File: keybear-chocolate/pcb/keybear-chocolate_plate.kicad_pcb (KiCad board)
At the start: 2 copper layers, 151.4 x 117.1 mm, 33 parts, among them J1 MJ-4PP-9, SW10 SW_PUSH, SW11 SW_PUSH, SW12 SW_PUSH, SW13 SW_PUSH, SW14 SW_PUSH, SW15 SW_PUSH, SW16 SW_PUSH, SW17 SW_PUSH, SW18 SW_PUSH, SW19 SW_PUSH, SW2 KEY_SWITCH, SW2 SW_PUSH, SW20 SW_PUSH, SW21 SW_PUSH, SW22 SW_PUSH, SW23 SW_PUSH, SW24 Rotary_Encoder_Switch, SW3 SW_PUSH, SW4 SW_PUSH, SW5 SW_PUSH, SW6 SW_PUSH, SW7 SW_PUSH, SW8 SW_PUSH, SW9 SW_PUSH, U1 ProMicro

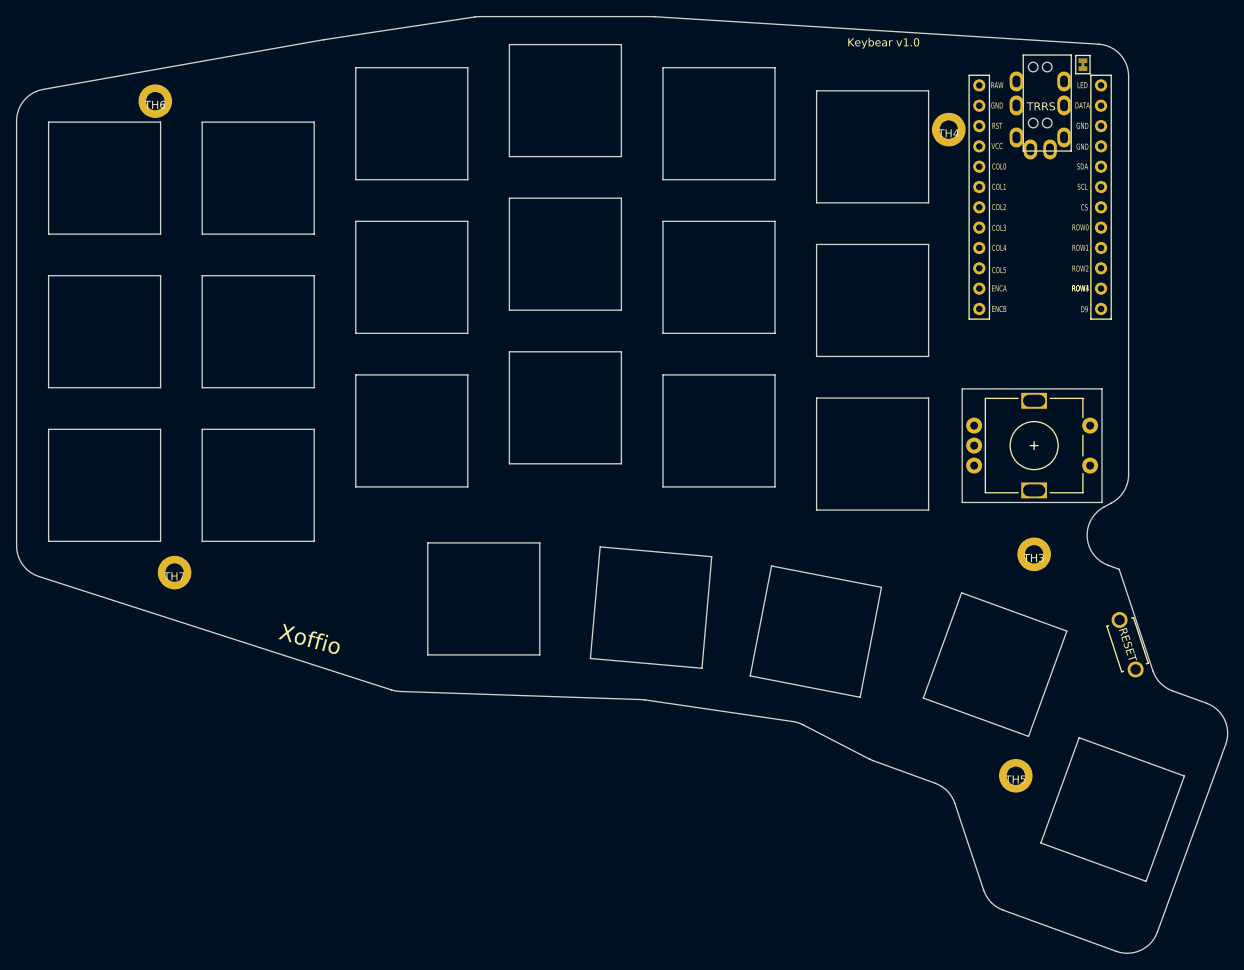
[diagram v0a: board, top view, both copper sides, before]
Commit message: updating the plate
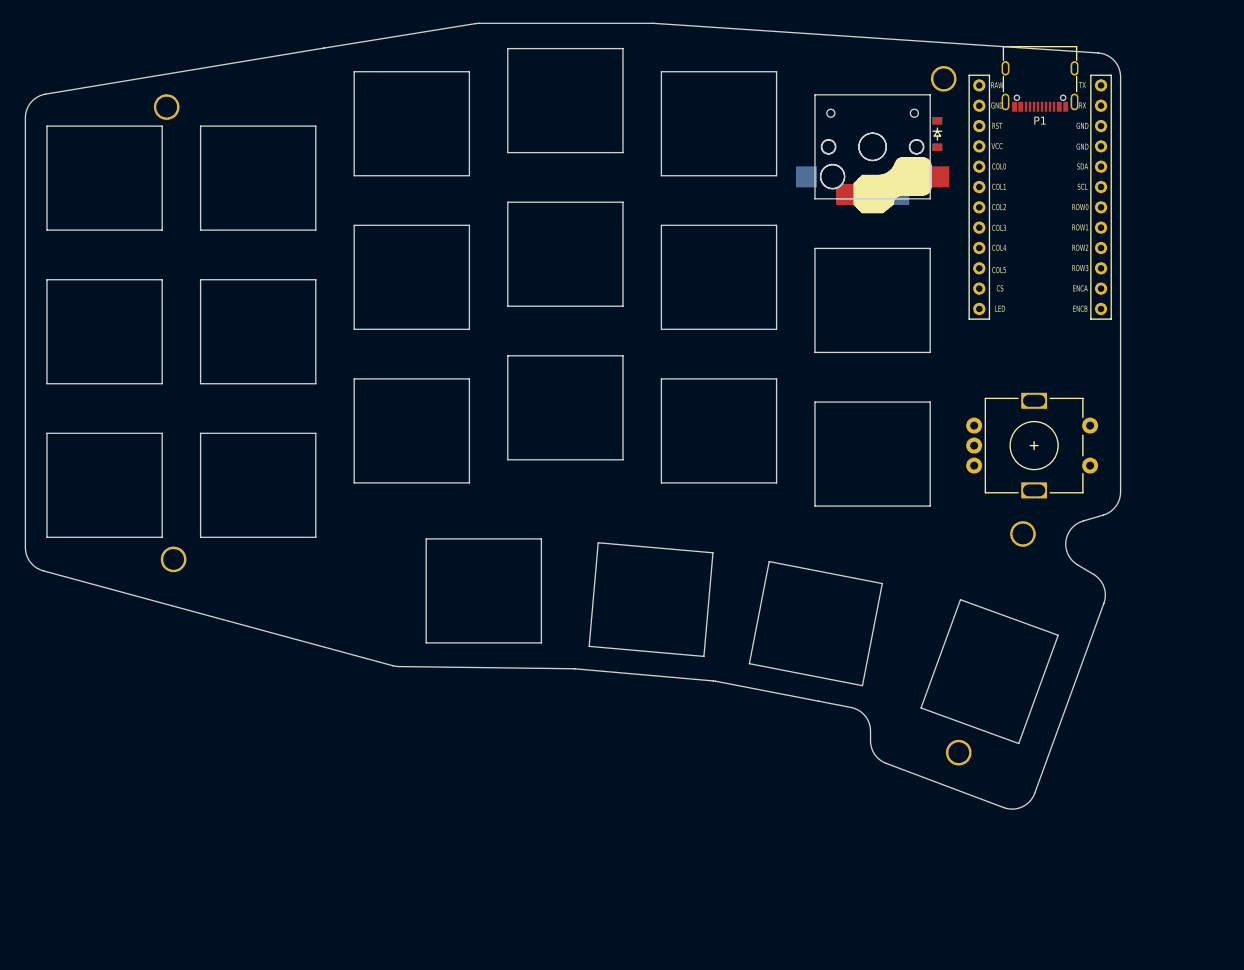
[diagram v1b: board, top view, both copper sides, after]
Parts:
- removed J1: MJ-4PP-9, kbd:MJ-4PP-9
- removed JP1: , kbd:JPC2
- removed RSW1: SW_PUSH, kbd:ResetSW
- removed SW10, SW11, SW12, SW13, SW14, SW15, SW16, SW17, SW18, SW19, SW2, SW20, SW21, SW22, SW23, SW3, SW4, SW5, SW7, SW8, SW9: SW_PUSH, kbd:SW_Hole
- removed SW2: KEY_SWITCH, kbd:SW_Hole
- removed TH3, TH4, TH5, TH6, TH7: HOLE, kbd:M2_Hole_TH
- added ?: , , F.Cu at (254.9, 99.2)
- added ?: , , F.Cu at (158.6, 159.3)
- added ?: , , F.Cu at (157.8, 102.7)
- added ?: , , F.Cu at (264.8, 156.1)
- added ?: , , F.Cu at (256.8, 183.4)
- added D18: , ComboDiode, F.Cu at (254.1, 106.1)
- added P1: USB_C_Plug, Connector_USB:USB_C_Receptacle_G-Switch_GT-USB-7010ASV, F.Cu at (266.9, 99.0)
- added S18: , PG1350, F.Cu at (246.0, 107.7)
- SW6: footprint kbd:SW_Hole -> kbd:Choc_Hotswap
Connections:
- SW24 pad A: ENCA -> (no net)
- SW24 pad B: ENCB -> (no net)
- SW24 pad C: GND -> (no net)
- SW24 pad S1: SW24A -> (no net)
- SW24 pad S2: SW24B -> (no net)
- U1 pad 1: LED -> (no net)
- U1 pad 10: row2 -> (no net)
- U1 pad 11: row3 -> (no net)
- U1 pad 12: unconnected-(U1-B5-Pad12) -> (no net)
- U1 pad 13: ENCB -> (no net)
- U1 pad 14: ENCA -> (no net)
- U1 pad 15: SW24A -> (no net)
- U1 pad 16: col4 -> (no net)
- U1 pad 17: col3 -> (no net)
- U1 pad 18: col2 -> (no net)
- U1 pad 19: col1 -> (no net)
- U1 pad 2: data -> (no net)
- U1 pad 20: col0 -> (no net)
- U1 pad 21: VCC -> (no net)
- U1 pad 22: reset -> (no net)
- U1 pad 23: GND -> (no net)
- U1 pad 24: RAW -> (no net)
- U1 pad 3: GND -> (no net)
- U1 pad 4: GND -> (no net)
- U1 pad 5: SDA -> (no net)
- U1 pad 6: SCL -> (no net)
- U1 pad 7: CS -> (no net)
- U1 pad 8: row0 -> (no net)
- U1 pad 9: row1 -> (no net)
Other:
- board size 151.4 x 117.1 mm -> 136.9 x 98.2 mm
- board text removed: "Keybear v1.0"
- board text removed: "Xoffio"
